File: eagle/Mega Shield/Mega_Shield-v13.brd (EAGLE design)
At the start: 143.5 x 95.2 mm, 40 parts, among them Q1 2N3904, Q2 2N3904, Q4 2N3904, Q5 2N3906

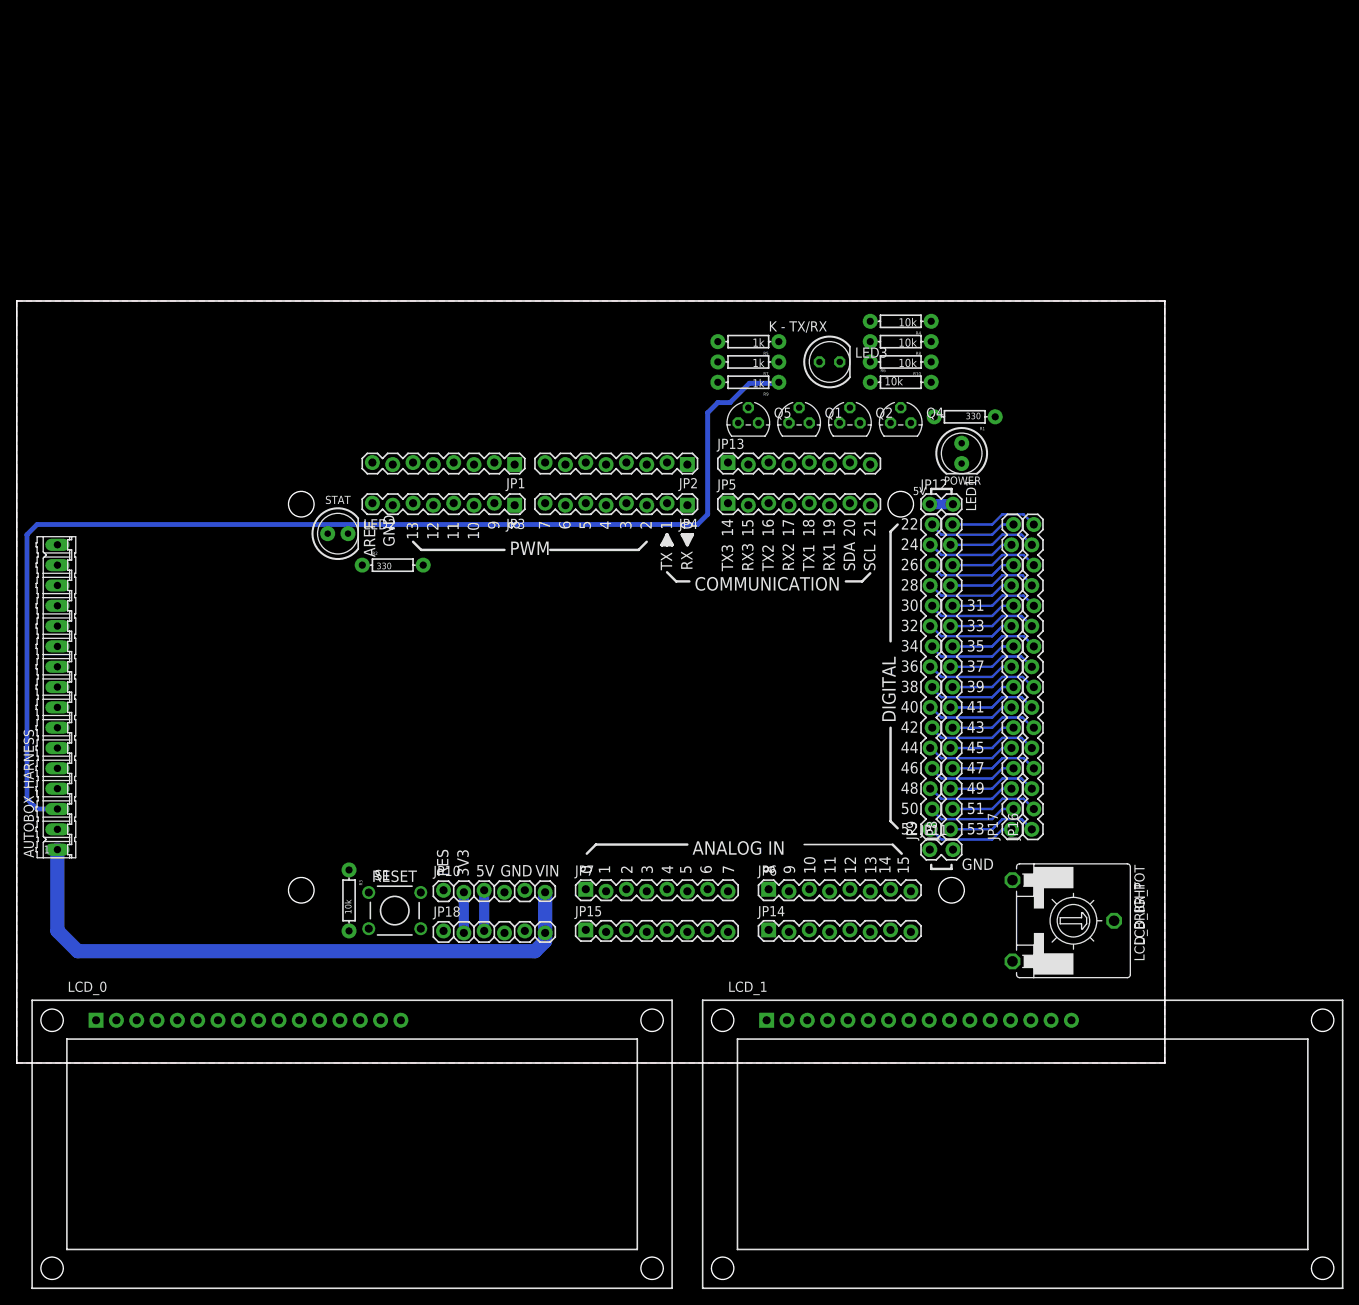
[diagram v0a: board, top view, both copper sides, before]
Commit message: did a lot of pcb work
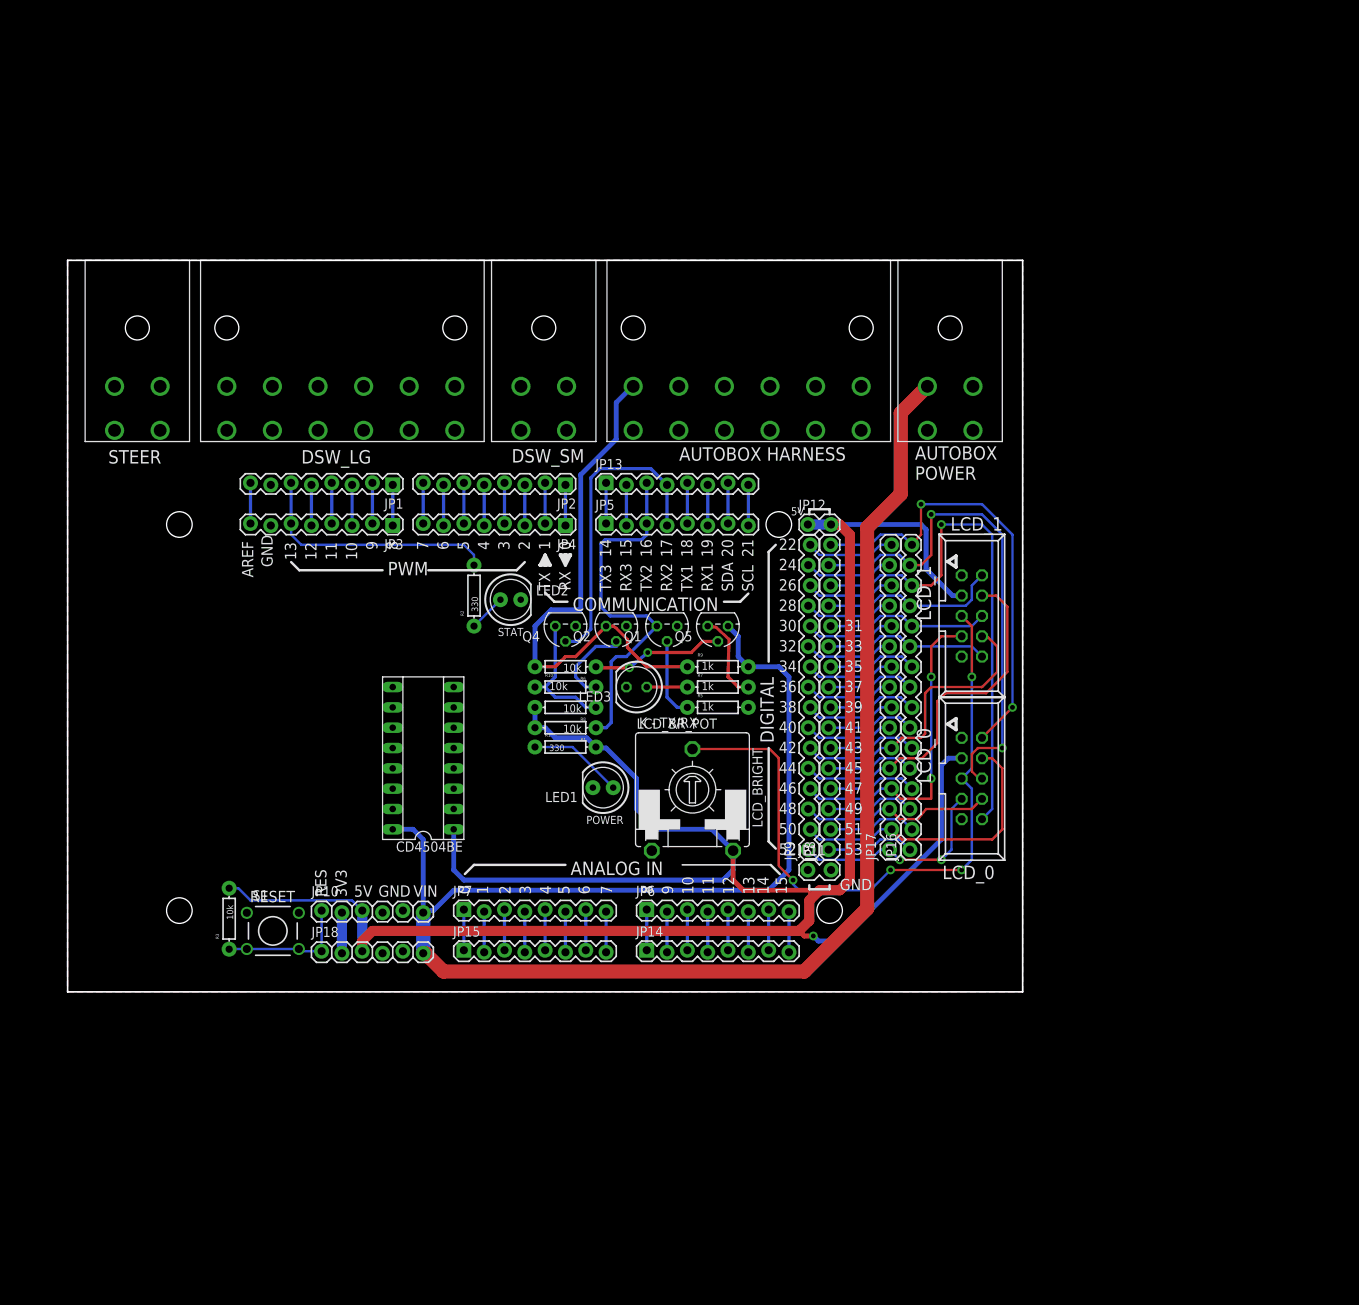
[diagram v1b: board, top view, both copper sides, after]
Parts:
- removed AUTOBOX_HARNESS: (no value), con-amp-quick:16P
- added ABOX_HARN, DSW_LG: (no value), Molex connectors:172064-0012
- added ABOX_PWR, DSW_SM, STEER: (no value), Molex connectors:172064-0004
- added CD4504BE: (no value), ic-package:SOCKET-16
- LCD_0, LCD_1: value LCD-16X2SILK -> 057-010-1; device SparkFun-Displays:LCD-16X2 -> con-panduit:057-010-1
- moved LCD_0 90.0 mm to (119.4, 35.6), turned to 270 degrees
- moved LCD_1 66.3 mm to (119.4, 55.9), turned to 270 degrees
- moved R4 65.9 mm to (68.6, 41.9)
- moved R1 64.8 mm to (68.6, 39.5), turned to 0 degrees
- moved R8 62.0 mm to (68.6, 44.5)
- moved LED1 61.3 mm to (73.3, 34.4), turned to 180 degrees
- moved R10 58.4 mm to (68.6, 47.0), turned to 0 degrees
- moved R6 55.0 mm to (68.6, 49.5), turned to 180 degrees
- moved LCD_BR_POT 50.4 mm to (84.5, 34.2), turned to 0 degrees
- moved Q4 49.0 mm to (68.6, 54.6), turned to 180 degrees
- moved LED3 47.3 mm to (77.5, 47.0), turned to 180 degrees
- moved R5 45.9 mm to (87.6, 44.5), turned to 0 degrees
- moved R7 40.8 mm to (87.6, 47.0), turned to 0 degrees
- moved Q2 38.7 mm to (74.9, 54.6), turned to 180 degrees
- moved R9 35.8 mm to (87.6, 49.5), turned to 0 degrees
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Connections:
- removed net 5V@1: JP12.1
- removed net A: LCD_0.15, LCD_1.15
- removed net K: LCD_0.16, LCD_1.16
- removed net N$3: Q1.1, R4.P$1
- new net N$11: CD4504BE.2
- new net N$12: CD4504BE.3
- new net N$13: CD4504BE.4
- new net N$14: CD4504BE.5
- new net N$15: CD4504BE.6
- new net N$16: CD4504BE.7
- new net N$19: CD4504BE.15
- new net N$20: CD4504BE.14
- new net N$22: CD4504BE.12
- new net N$23: CD4504BE.11
- new net N$24: CD4504BE.10
- new net N$25: CD4504BE.9
- net 5V: now also CD4504BE.1, JP12.1, LCD_0.3, LCD_1.3; no longer LCD_0.2, LCD_1.2
- net D19: now also Q1.1, R4.P$1; no longer Q1.3
- net D22: now also LCD_0.7; no longer LCD_0.4
- net D23: now also LCD_0.2; no longer LCD_0.6
- net D24: now also LCD_0.4; no longer LCD_0.11
- net D25: now also LCD_0.6; no longer LCD_0.12
- net D26: now also LCD_0.8; no longer LCD_0.13
- net D27: now also LCD_0.10; no longer LCD_0.14
- net D28: now also LCD_1.7; no longer LCD_1.4
- net D29: now also LCD_1.2; no longer LCD_1.6
- net D30: now also LCD_1.4; no longer LCD_1.11
- net D31: now also LCD_1.6; no longer LCD_1.12
- net D32: now also LCD_1.8; no longer LCD_1.13
- net D33: now also LCD_1.10; no longer LCD_1.14
- net GND: now also ABOX_PWR.CKT2, CD4504BE.13, CD4504BE.8, LCD_0.9, LCD_1.9, Q1.3; no longer AUTOBOX_HARNESS.2, LCD_0.5, LCD_1.5
- net LCD_BR: now also LCD_0.5, LCD_1.5; no longer LCD_0.3, LCD_1.3
- net MODE0: now also ABOX_HARN.CKT6; no longer AUTOBOX_HARNESS.8
- net MODE1: now also ABOX_HARN.CKT7; no longer AUTOBOX_HARNESS.9
- net N$1: now also ABOX_HARN.CKT12; no longer AUTOBOX_HARNESS.16
- net N$2: now also ABOX_HARN.CKT11; no longer AUTOBOX_HARNESS.15
- net SERIAL_K: now also ABOX_HARN.CKT1; no longer AUTOBOX_HARNESS.3
- net SERIAL_L: now also ABOX_HARN.CKT2; no longer AUTOBOX_HARNESS.4
- net SHFT_D: now also ABOX_PWR.CKT4; no longer AUTOBOX_HARNESS.14
- net SHFT_U: now also ABOX_PWR.CKT3; no longer AUTOBOX_HARNESS.13
- net SW1: now also ABOX_HARN.CKT3; no longer AUTOBOX_HARNESS.5
- net SW2: now also ABOX_HARN.CKT4; no longer AUTOBOX_HARNESS.6
- net SW3: now also ABOX_HARN.CKT5; no longer AUTOBOX_HARNESS.7
- net TRC_POT: now also ABOX_HARN.CKT10; no longer AUTOBOX_HARNESS.12
- net TRC_SW0: now also ABOX_HARN.CKT8; no longer AUTOBOX_HARNESS.10
- net TRC_SW1: now also ABOX_HARN.CKT9; no longer AUTOBOX_HARNESS.11
- net VIN: now also ABOX_PWR.CKT1, CD4504BE.16; no longer AUTOBOX_HARNESS.1
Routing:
- net 5V: track 7.80 -> 292.4 mm, vias 0 -> 1
- net VIN: track 79.0 -> 230.4 mm
- net LCD_BR: track 0.00 -> 84.1 mm, vias 0 -> 4
- net SERIAL_K: track 146.7 -> 66.1 mm
- net D27: track 11.2 -> 64.7 mm, vias 0 -> 1
- net D25: track 11.2 -> 64.0 mm, vias 0 -> 2
- net D19: track 0.13 -> 45.9 mm
- net D23: track 11.2 -> 56.8 mm, vias 0 -> 2
- net D18: track 0.13 -> 38.8 mm
- net D30: track 11.2 -> 45.9 mm
- net D13: track 0.00 -> 31.7 mm
- net D28: track 11.3 -> 40.2 mm, vias 0 -> 2
- net D32: track 11.3 -> 37.0 mm
- net D24: track 11.3 -> 36.9 mm
- net N$10: track 0.00 -> 16.8 mm
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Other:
- board size 143.5 x 95.2 mm -> 119.4 x 91.4 mm
- board text added: "AUTOBOX HARNESS"
- board text added: "AUTOBOX POWER"
- board text added: "DSW_LG"
- board text added: "DSW_SM"
- board text added: "STEER"

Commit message: lots of board work
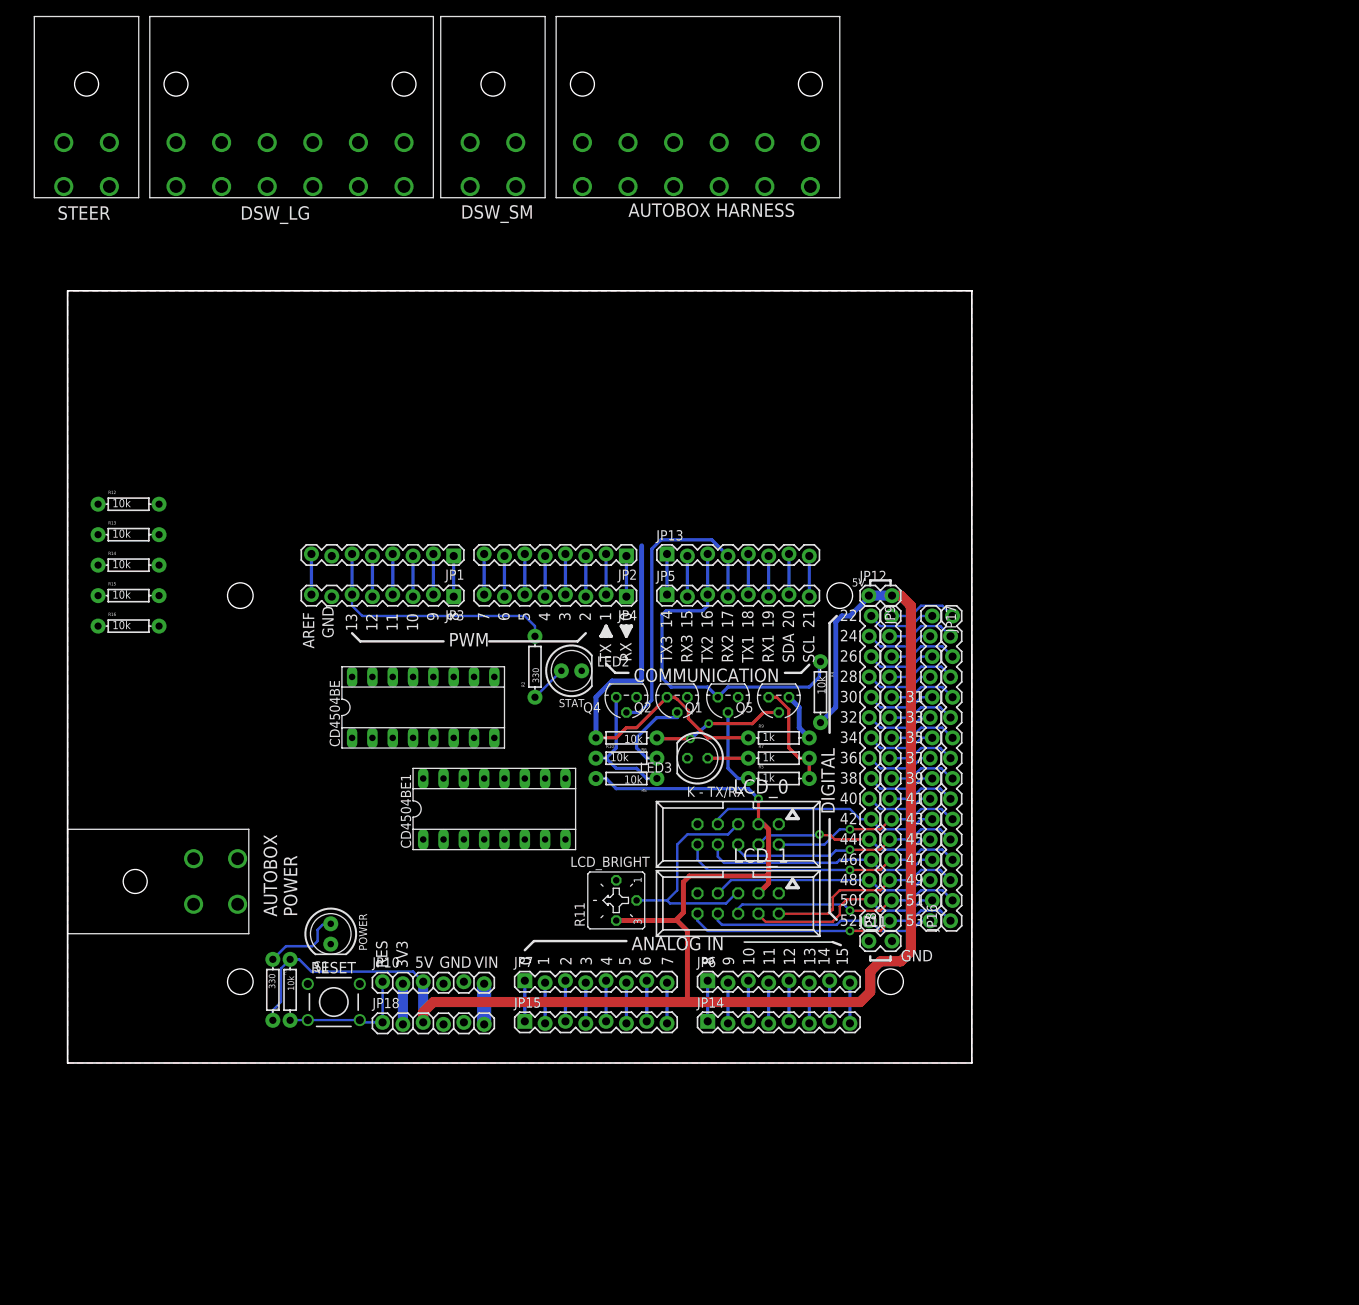
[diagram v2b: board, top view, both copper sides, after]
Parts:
- removed LCD_BR_POT: (no value), pot:CA14V
- added CD4504BE1: (no value), ic-package:SOCKET-16
- added R11: (no value), pot:CT6
- added R12, R13, R14, R15, R16: 10k, SparkFun-Passives:AXIAL-0.3EZ
- moved ABOX_PWR 136.8 mm to (6.35, 29.2), turned to 270 degrees
- moved R1 47.5 mm to (32.0, 9.14), turned to 270 degrees
- moved LCD_1 46.3 mm to (90.2, 19.9), turned to 180 degrees
- moved LED1 38.6 mm to (39.2, 16.1), turned to 270 degrees
- moved R4 32.2 mm to (100.5, 46.4), turned to 270 degrees
- moved ABOX_HARN 31.1 mm to (102.9, 130.8)
- moved DSW_LG 31.1 mm to (52.1, 130.8)
- moved DSW_SM 31.1 mm to (66.0, 130.8)
- moved STEER 31.1 mm to (15.2, 130.8)
- moved JP9 30.2 mm to (106.7, 55.9), turned to 270 degrees
- moved LCD_0 30.0 mm to (90.2, 28.6), turned to 180 degrees
- moved JP17 29.6 mm to (114.3, 55.9), turned to 270 degrees
- moved JP12 11.7 mm to (106.7, 58.4)
- moved JP13 11.7 mm to (81.3, 63.5)
- moved JP14 11.7 mm to (86.4, 5.08)
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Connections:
- removed net N$1: ABOX_HARN.CKT12
- removed net N$11: CD4504BE.2
- removed net N$12: CD4504BE.3
- removed net N$13: CD4504BE.4
- removed net N$14: CD4504BE.5
- removed net N$15: CD4504BE.6
- removed net N$16: CD4504BE.7
- removed net N$2 (its old number): ABOX_HARN.CKT11
- removed net N$24: CD4504BE.10
- removed net N$25: CD4504BE.9
- removed net TRC_POT: ABOX_HARN.CKT10
- removed net TRC_SW0: ABOX_HARN.CKT8
- removed net TRC_SW1: ABOX_HARN.CKT9
- new net LAUNCHSW_12: CD4504BE.3, DSW_LG.CKT2, R13.P$2
- new net LAUNCHSW_LED: CD4504BE1.2, DSW_LG.CKT3
- new net LAUNCH_LED: ABOX_HARN.CKT11, CD4504BE1.3
- new net LAUNCH_SW: ABOX_HARN.CKT8, CD4504BE.2
- new net N$27: CD4504BE1.6
- new net N$28: CD4504BE1.7
- new net N$29: DSW_SM.CKT4
- new net N$32: CD4504BE1.15
- new net N$33: CD4504BE1.14
- new net N$35: CD4504BE1.12
- new net N$36: CD4504BE1.11
- new net N$37: CD4504BE1.10
- new net N$38: CD4504BE1.9
- new net N$97: DSW_SM.CKT3
- new net N$98: DSW_SM.CKT2
- new net N$99: DSW_SM.CKT1
- new net TRAC_LED: ABOX_HARN.CKT12, CD4504BE1.5
- new net TRA_CTL_LED: CD4504BE1.4, DSW_LG.CKT5
- new net TRA_CTL_POT: ABOX_HARN.CKT10, DSW_LG.CKT7
- new net TRA_CTL_SW: ABOX_HARN.CKT9, CD4504BE.4
- new net TRA_CTL_SW_12: CD4504BE.5, DSW_LG.CKT4, R14.P$2
- net 5V: now also CD4504BE.16, CD4504BE1.1, R11.E, R12.P$1; no longer CD4504BE.1, LCD_BR_POT.E
- net D22: now also CD4504BE.6; no longer LCD_0.7
- net D23: now also CD4504BE.10; no longer LCD_0.2
- net D24: now also DSW_LG.CKT6, R12.P$2; no longer LCD_0.4
- net D25: no longer LCD_0.6
- net D26: no longer LCD_0.8
- net D27: no longer LCD_0.10
- net D28: no longer LCD_1.7
- net D29: no longer LCD_1.2
- net D30: no longer LCD_1.4
- net D31: no longer LCD_1.6
- net D32: no longer LCD_1.8
- net D33: no longer LCD_1.10
- net D42: now also LCD_0.7
- net D43: now also LCD_0.2
- net D44: now also LCD_0.4
- net D45: now also LCD_0.6
- net D46: now also LCD_0.8
- net D47: now also LCD_0.10
- net D48: now also LCD_1.7
- net D49: now also LCD_1.2
- net D50: now also LCD_1.4
- net D51: now also LCD_1.6
- net D52: now also LCD_1.8
- net D53: now also LCD_1.10
- net GND: now also CD4504BE1.13, CD4504BE1.8, R11.A, R13.P$1, R14.P$1, R15.P$2, R16.P$1, STEER.CKT2; no longer LCD_BR_POT.A
- net LCD_BR: now also R11.S; no longer LCD_BR_POT.S
- net MODE0: now also DSW_LG.CKT8
- net MODE1: now also DSW_LG.CKT9
- net SHFT_D: now also CD4504BE.9, R16.P$2, STEER.CKT4
- net SHFT_U: now also CD4504BE.7, R15.P$1, STEER.CKT3
- net SW1: now also DSW_LG.CKT10
- net SW2: now also DSW_LG.CKT11
- net SW3: now also DSW_LG.CKT12
- net VIN: now also CD4504BE.1, CD4504BE1.16, DSW_LG.CKT1, STEER.CKT1; no longer CD4504BE.16
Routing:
- net VIN: track 230.4 -> 11.2 mm
- net D27: track 64.7 -> 8.67 mm, vias 1 -> 0
- net D25: track 64.0 -> 8.67 mm, vias 2 -> 0
- net LCD_BR: track 84.1 -> 29.6 mm, vias 4 -> 0
- net 5V: track 292.4 -> 243.4 mm
- net D23: track 56.8 -> 8.67 mm, vias 2 -> 0
- net D30: track 45.9 -> 8.75 mm
- net D28: track 40.2 -> 8.67 mm, vias 2 -> 0
- net D32: track 37.0 -> 8.67 mm
- net D24: track 36.9 -> 8.55 mm
- net D47: track 11.2 -> 35.9 mm, vias 0 -> 1
- net D53: track 11.2 -> 34.7 mm, vias 0 -> 1
- net D46: track 11.2 -> 29.9 mm
- net D42: track 11.2 -> 29.6 mm
- net D51: track 11.2 -> 29.5 mm, vias 0 -> 1
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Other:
- board size 119.4 x 91.4 mm -> 113 x 96.5 mm
- board text removed: "LCD_0"
- board text removed: "LCD_1"
